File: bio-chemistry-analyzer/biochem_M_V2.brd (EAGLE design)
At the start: 87.1 x 100 mm, 37 parts, among them J1 61201021621, J2 USB1135-15-9-L-B_REVA1, Q4-T IRFZ44N, Q4-T4 IRFZ44N, Q4-T5 IRFZ44N, Q4-T6 IRFZ44N

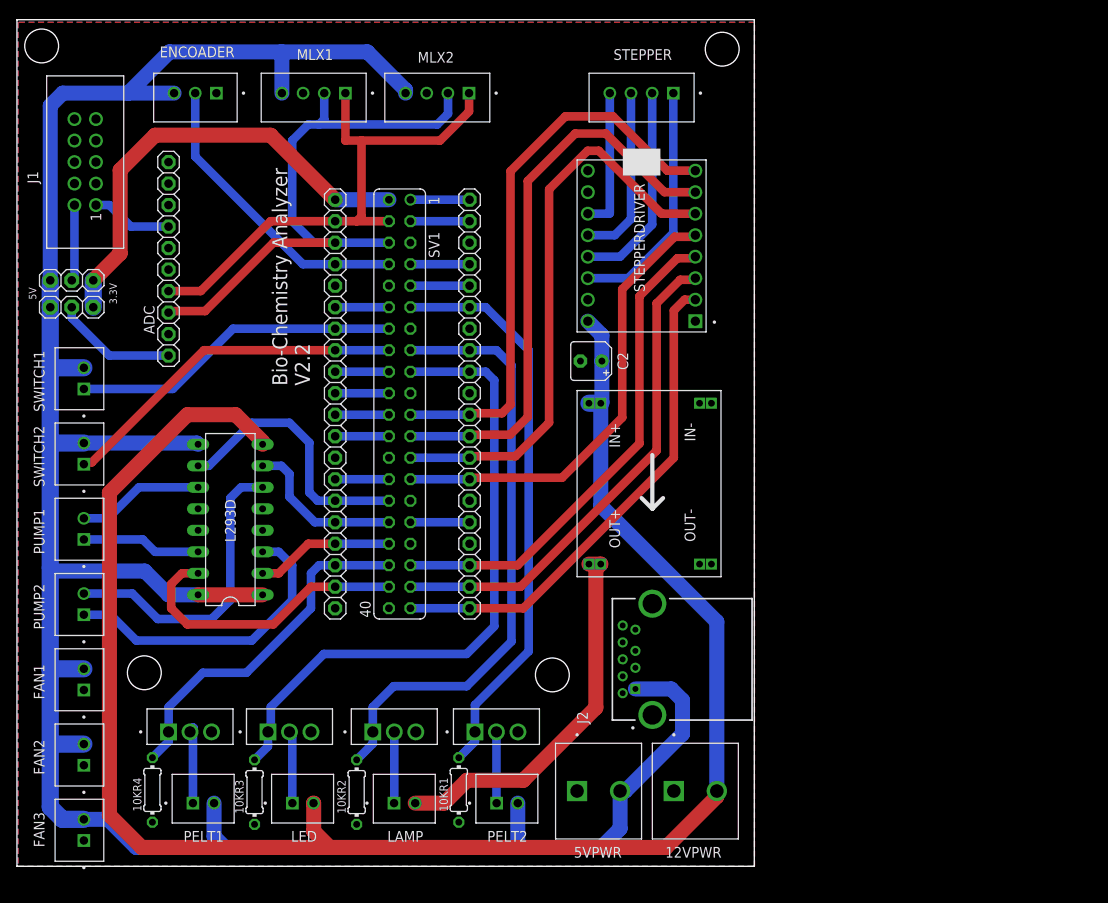
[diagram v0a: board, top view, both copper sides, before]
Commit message: PCB Changes
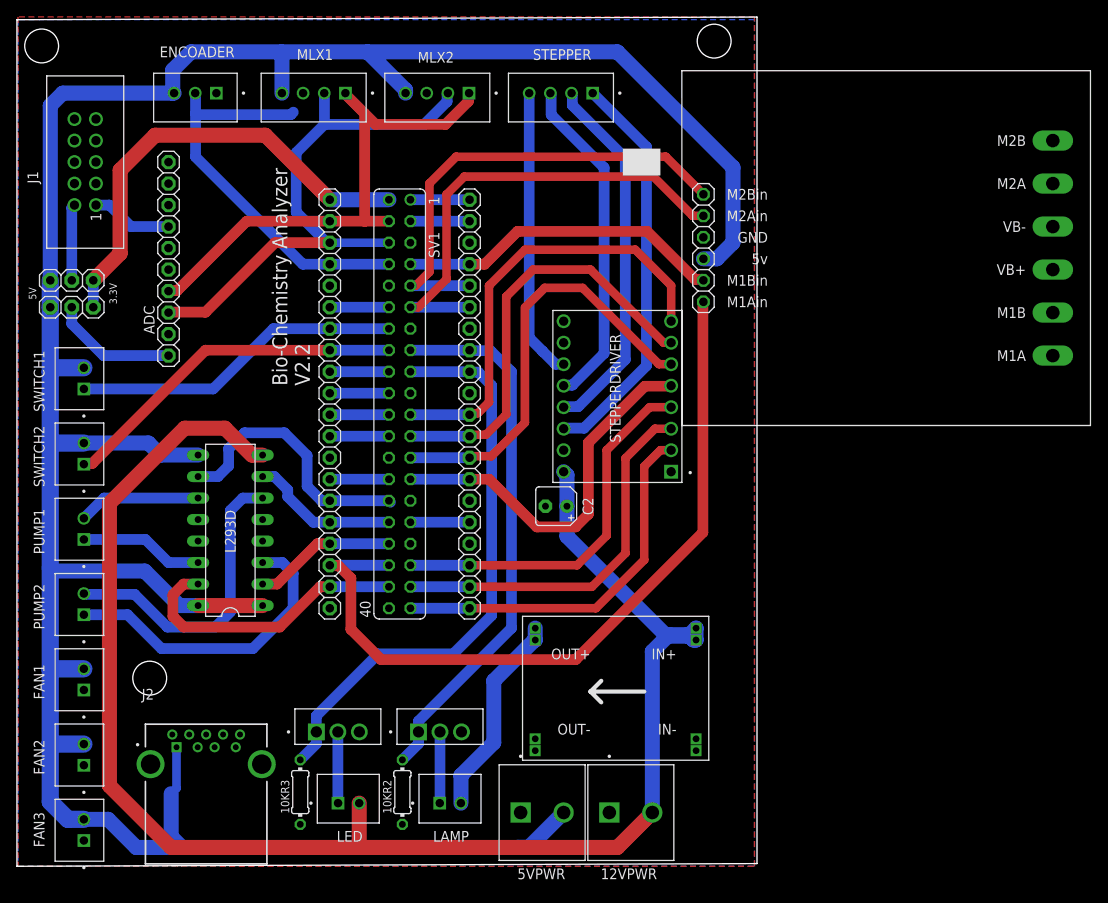
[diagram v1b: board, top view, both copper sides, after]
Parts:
- removed 10KR1, 10KR4: (no value), rcl:0204/7
- removed PELT1, PELT2: B4B-XH-2PIN2PIN, B4B-XH-A_LF__SN_:B4BXH2
- removed Q4-T5, Q4-T6: IRFZ44N, IRFZ44N:TO254P1016X419X2286-3
- added U$2: MDD3A, MDD3A:FOOTPRINT
- moved J2 54.1 mm to (22.2, 12.1), turned to 0 degrees
- moved U$1 30.9 mm to (81.6, 29.5), turned to 180 degrees
- moved STEPPERDRIVER 18.0 mm to (70.8, 55.5)
- moved C2 17.6 mm to (63.6, 42.5)
- moved STEPPER 9.52 mm to (64.1, 90.8)
- moved 12VPWR 8.03 mm to (69.8, 6.35)
- moved 5VPWR 7.13 mm to (59.4, 6.35)
- moved Q4-T4 5.71 mm to (37.8, 15.9)
- moved 10KR2 5.40 mm to (45.4, 8.76)
- moved LAMP 5.40 mm to (51.2, 6.99)
- moved LED 5.40 mm to (39.2, 6.99)
- moved 10KR3 5.40 mm to (33.3, 8.76)
- moved Q4-T 5.40 mm to (49.8, 15.9)
- moved L293D 1.27 mm to (25.1, 39.7)
- moved JP2 0.64 mm to (36.8, 54.6)
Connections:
- removed net N$3: JP1.4, SV1.7
- removed net N$6: JP1.5, SV1.9
- removed net PELT1: 10KR4.2, JP2.3, Q4-T5.1, SV1.36
- removed net PELT2: 10KR1.2, JP1.6, Q4-T6.1, SV1.11
- removed net PELTIER1: PELT1.1, Q4-T5.2
- removed net PELTIER2: PELT2.1, Q4-T6.2
- new net PELT1A: JP2.3, SV1.36, U$2.M1AIN
- new net PELT1B: JP1.4, SV1.7, U$2.M1BIN
- new net PELT2A: JP1.6, SV1.11, U$2.M2AIN
- new net PELT2B: JP1.5, SV1.9, U$2.M2BIN
- net 5V: now also U$2.5V; no longer PELT1.2, PELT2.2
- net GND: now also U$2.GND; no longer 10KR1.1, 10KR4.1, Q4-T5.3, Q4-T6.3
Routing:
- net PELT1A: track 0.00 -> 92.7 mm
- net PELT2: track 67.6 -> 0.00 mm
- net PELT2B: track 0.00 -> 55.9 mm
- net PELT2A: track 0.00 -> 55.8 mm
- net PELT1: track 42.2 -> 0.00 mm
- net PELT1B: track 0.00 -> 38.6 mm
- net 5V: track 302.2 -> 338.7 mm
- net 12V: track 207.5 -> 185.5 mm
- net 6V: track 44.6 -> 24.4 mm
- net B1: track 24.7 -> 43.7 mm
- net A1: track 20.8 -> 39.7 mm
- net B2: track 28.8 -> 47.7 mm
- net A2: track 16.8 -> 34.3 mm
- net STEPSLP: track 67.9 -> 50.8 mm
- net STEPSTP: track 67.7 -> 50.7 mm
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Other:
- board size 87.1 x 100 mm -> 87.4 x 100.3 mm
